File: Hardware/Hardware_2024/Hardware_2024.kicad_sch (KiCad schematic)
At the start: 51 parts, among them U1 Raspberry_Pi, U2 SHHD003A0A, U3 MCP3008

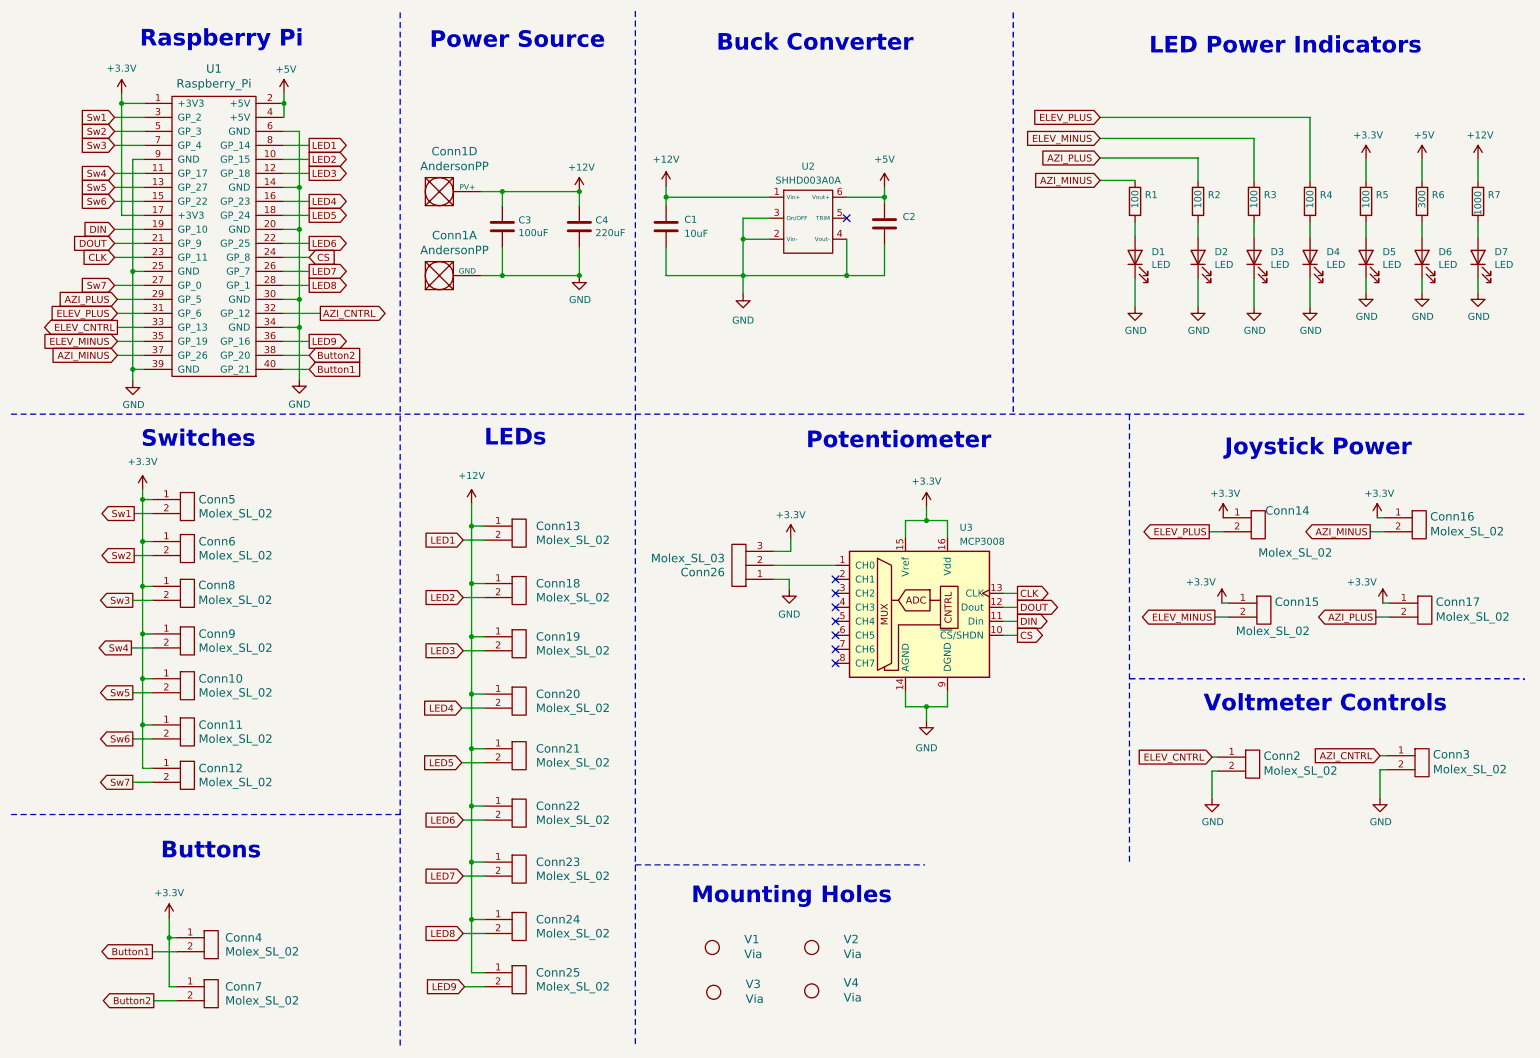
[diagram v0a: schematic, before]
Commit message: Updated with changes
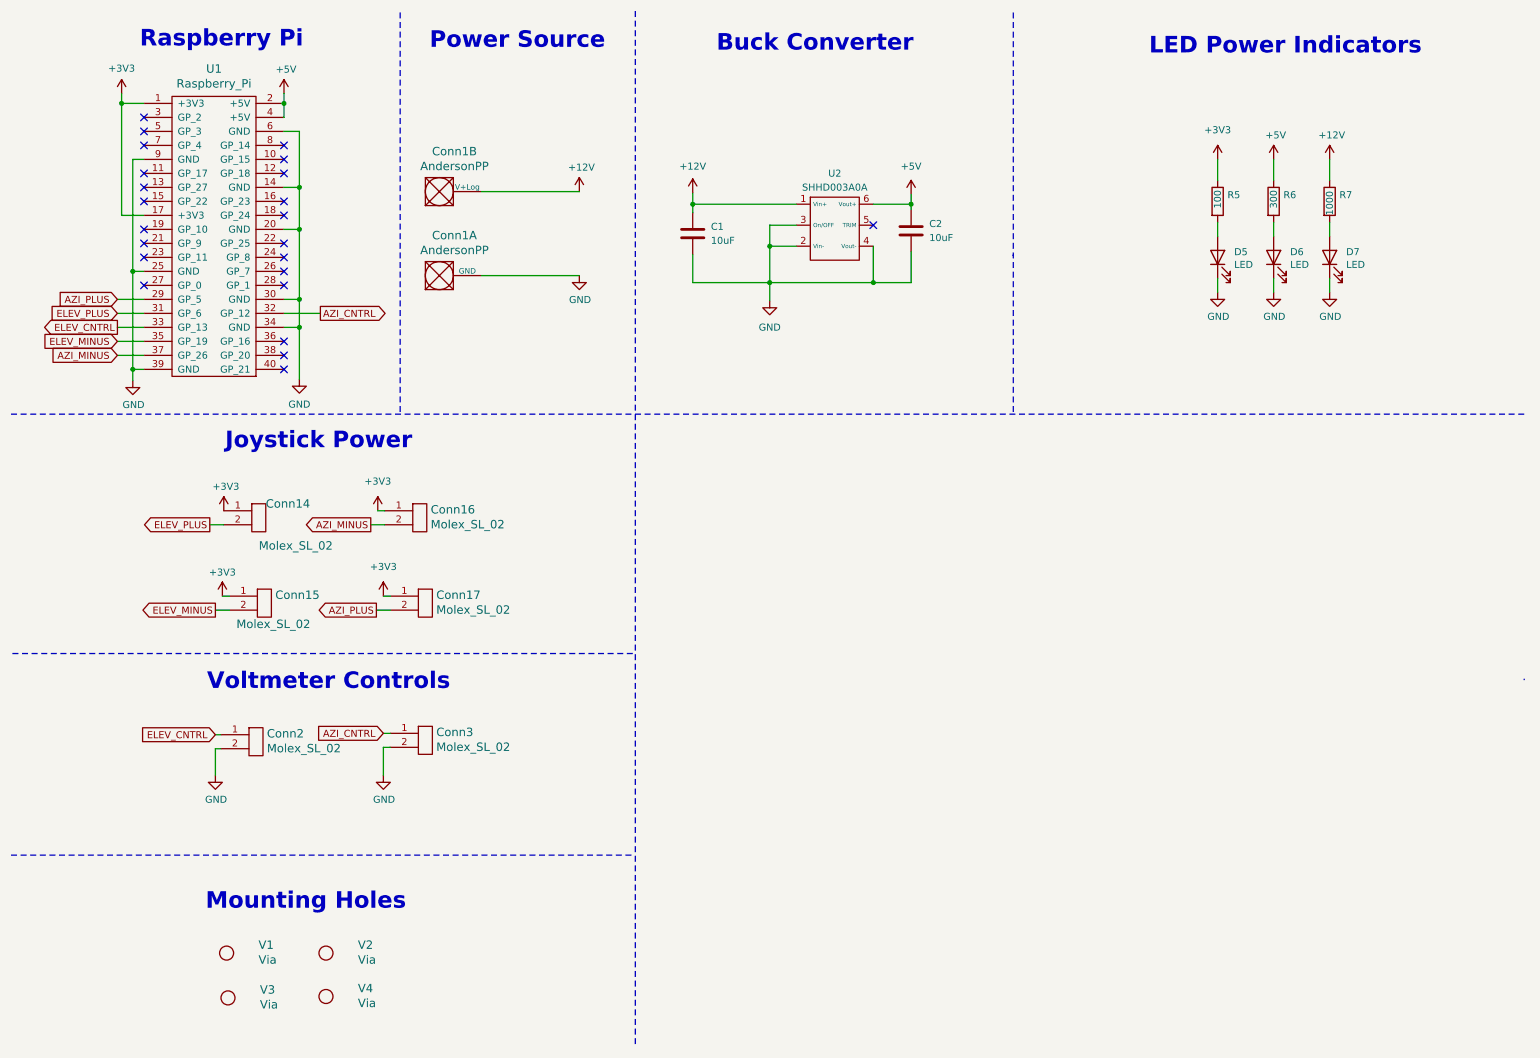
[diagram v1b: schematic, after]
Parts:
- removed C3: 100uF, Capacitor_THT:CP_Radial_D6.3mm_P2.50mm, symbol Device:C
- removed C4: 220uF, Capacitor_THT:CP_Radial_D6.3mm_P2.50mm, symbol Device:C
- removed Conn10, Conn11, Conn12, Conn13, Conn18, Conn19, Conn20, Conn21, Conn22, Conn23, Conn24, Conn25, Conn4, Conn5, Conn6, Conn7, Conn8, Conn9: Molex_SL_02, MRDT_Connectors:MOLEX_SL_02_Vertical, symbol MRDT_Connectors:Molex_SL_02
- removed Conn26: Molex_SL_03, MRDT_Connectors:MOLEX_SL_03_Vertical, symbol MRDT_Connectors:Molex_SL_03
- removed D1, D2, D3, D4: LED, LED_SMD:LED_0603_1608Metric_Pad1.05x0.95mm_HandSolder, symbol Device:LED
- removed R1, R2, R3, R4: 100, Resistor_SMD:R_0603_1608Metric_Pad0.98x0.95mm_HandSolder, symbol Device:R
- removed U3: MCP3008, Package_DIP:DIP-16_W7.62mm, symbol Analog_ADC:MCP3008
- Conn1: footprint MRDT_Connectors:Square_Anderson_2_H_Stacked -> MRDT_Connectors:Square_Anderson_2_H_Side_By_Side
- U1: footprint MRDT_Shields:RASPBERRY_PI_HEADERS -> MRDT_Shields:RaspberryPi_THT_BOTTOM
- U2: footprint SHHD003A04A41:SHHD003A0A-SRZ -> MRDT_Devices:SHHD003A0A41Z_Through_Hole
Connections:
- net +3.3V is gone; now on net +3V3: U1.1 (+3V3), U1.17 (+3V3)
- net +12V: now also Conn1.2 (V+Log); no longer Conn1.4 (PV+)
- net Button1: no longer names the net of U1.40 (GP_21)
- net Button2: no longer names the net of U1.38 (GP_20)
- net CLK: no longer names the net of U1.23 (GP_11)
- net CS: no longer names the net of U1.24 (GP_8)
- net DIN: no longer names the net of U1.19 (GP_10)
- net DOUT: no longer names the net of U1.21 (GP_9)
- net LED1: no longer names the net of U1.8 (GP_14)
- net LED2: no longer names the net of U1.10 (GP_15)
- net LED3: no longer names the net of U1.12 (GP_18)
- net LED4: no longer names the net of U1.16 (GP_23)
- net LED5: no longer names the net of U1.18 (GP_24)
- net LED6: no longer names the net of U1.22 (GP_25)
- net LED7: no longer names the net of U1.26 (GP_7)
- net LED8: no longer names the net of U1.28 (GP_1)
- net LED9: no longer names the net of U1.36 (GP_16)
- net Sw1: no longer names the net of U1.3 (GP_2)
- net Sw2: no longer names the net of U1.5 (GP_3)
- net Sw3: no longer names the net of U1.7 (GP_4)
- net Sw4: no longer names the net of U1.11 (GP_17)
- net Sw5: no longer names the net of U1.13 (GP_27)
- net Sw6: no longer names the net of U1.15 (GP_22)
- net Sw7: no longer names the net of U1.27 (GP_0)
- no-connect marks 8 -> 23
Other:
- note removed: "Buttons"
- note removed: "LEDs"
- note removed: "Potentiometer"
- note removed: "Switches"
- moved on the sheet: C1, C2, Conn14, Conn15, Conn16, Conn17, Conn2, Conn3, D5, D6, D7, R5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
